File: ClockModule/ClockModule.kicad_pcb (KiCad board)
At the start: 2 copper layers, 93.5 x 65.5 mm, 34 parts, among them J1 Conn_01x05_Pin, SW1 SW_SPDT, U1 LM555xN, U2 LM555xN, U3 OR, U4 NOT, U6 LM555xN

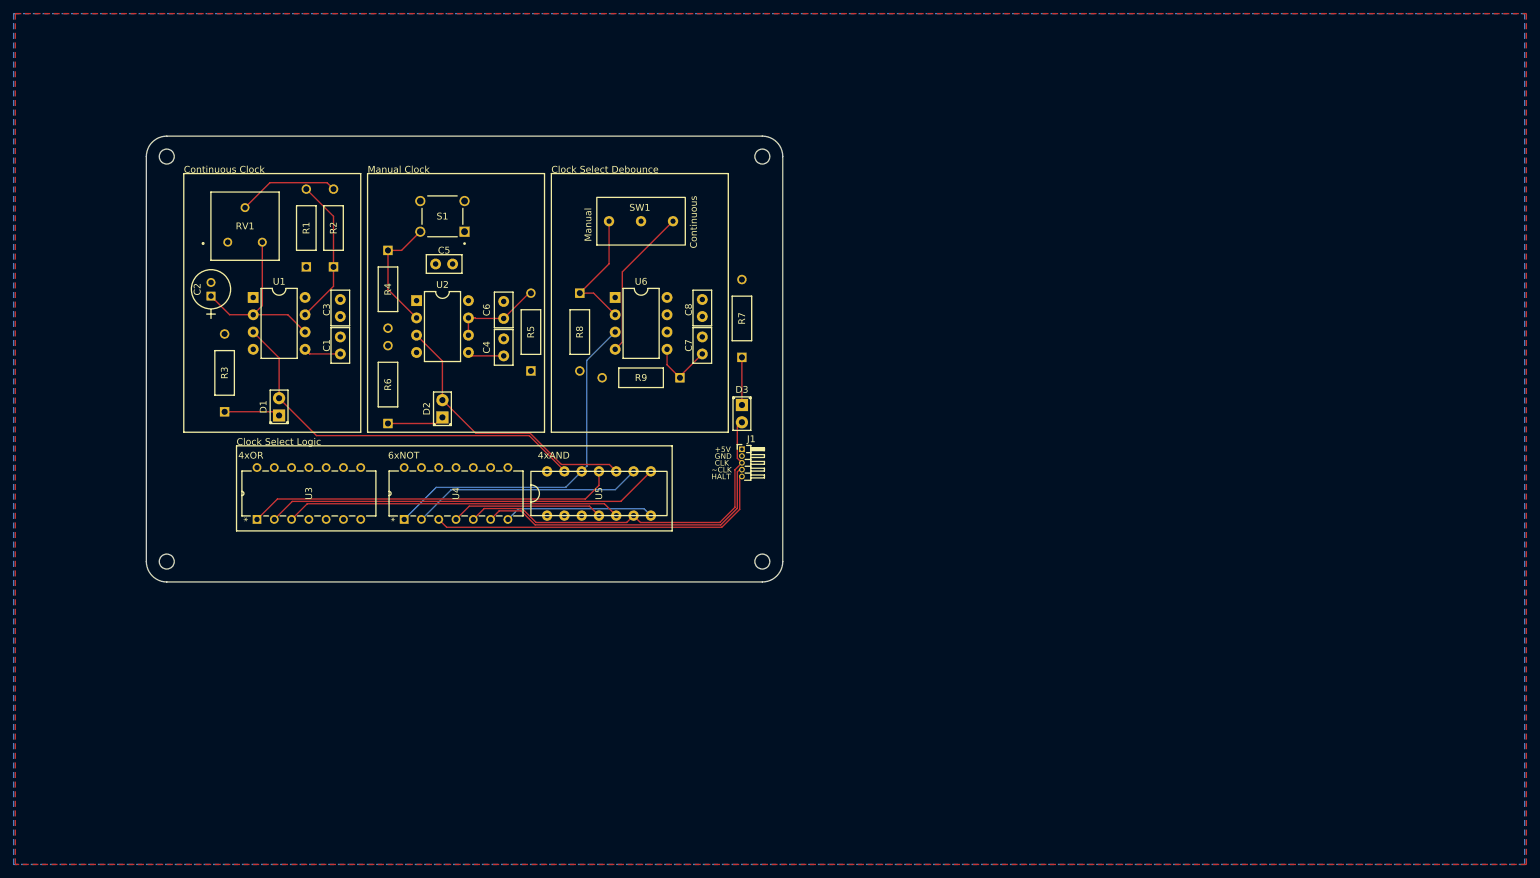
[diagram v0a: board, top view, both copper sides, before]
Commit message: Final clock updates
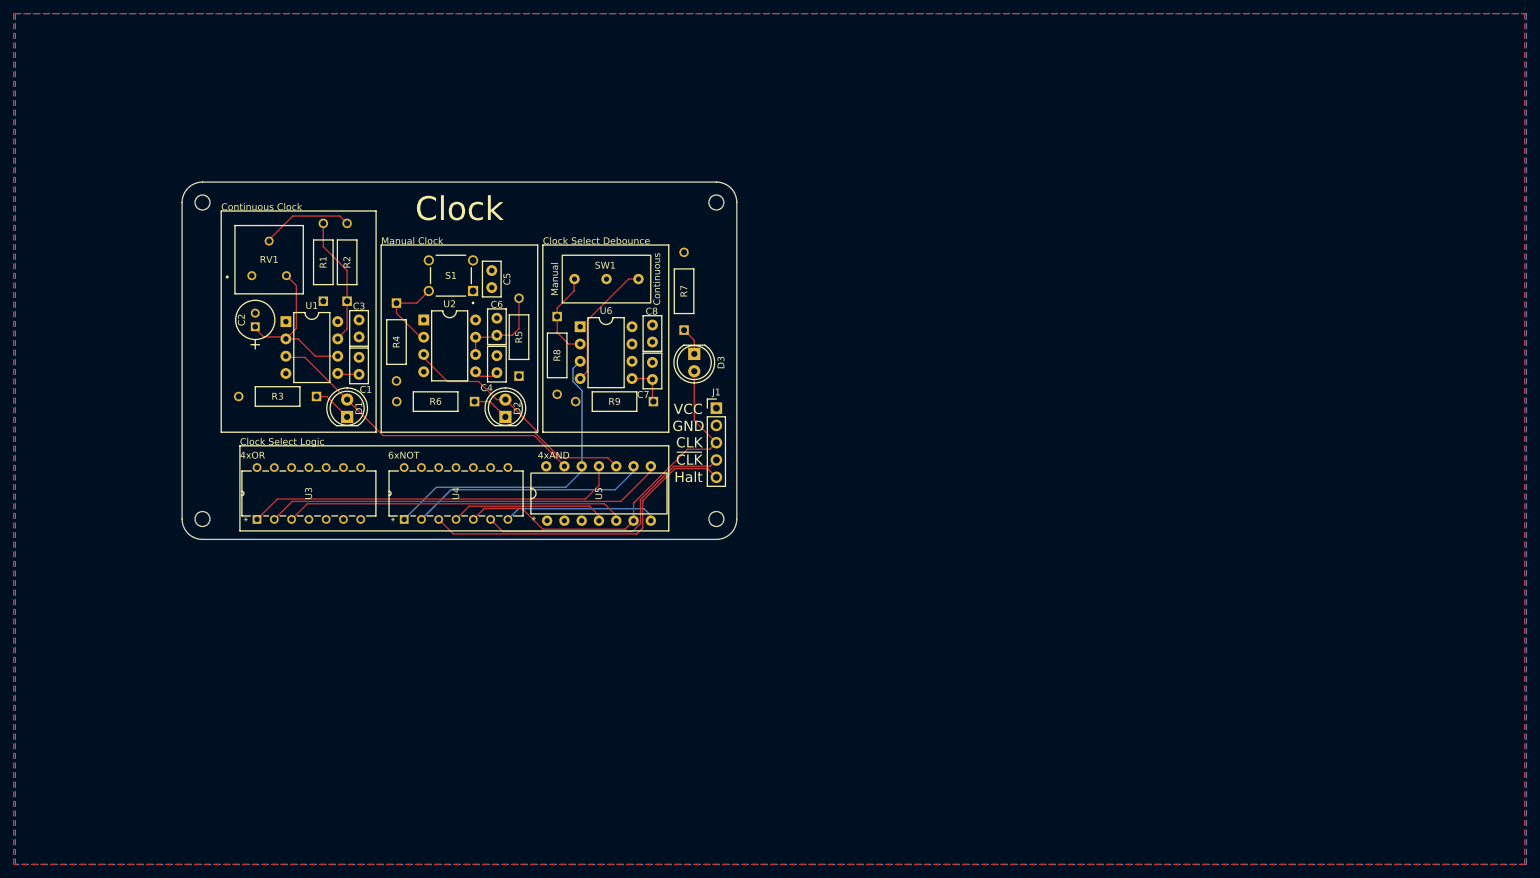
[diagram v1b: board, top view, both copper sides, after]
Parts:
- D1, D2, D3: footprint LED_THT:LED_D2.0mm_W4.8mm_H2.5mm_FlatTop -> LED_THT:LED_D5.0mm
- J1: footprint Connector_PinHeader_1.00mm:PinHeader_1x05_P1.00mm_Horizontal -> Connector_PinHeader_2.54mm:PinHeader_1x05_P2.54mm_Vertical
- moved R3 13.7 mm to (77.5, 102.8), turned to 180 degrees
- moved R6 13.1 mm to (100.7, 103.5), turned to 180 degrees
- moved D3 10.3 mm to (133.0, 96.5)
- moved D1 10.0 mm to (82.0, 105.8)
- moved SW1 9.90 mm to (120.1, 85.5)
- moved REF** 9.55 mm to (136.2, 74.2)
- moved R7 9.39 mm to (131.5, 93.0)
- moved D2 9.25 mm to (105.2, 105.8)
- moved REF** 9.20 mm to (136.2, 120.8)
- moved S1 8.80 mm to (97.2, 85.0)
- moved REF** 8.55 mm to (60.8, 74.2)
- moved C7 8.23 mm to (126.9, 100.2)
- moved C8 8.23 mm to (126.9, 92.2)
- moved REF** 8.16 mm to (60.8, 120.8)
- moved C2 7.91 mm to (68.5, 92.5)
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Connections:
- J1 pad 1: GND -> +5V
- J1 pad 2: +5V -> GND
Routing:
- net /AstableClock/CLK: track 57.7 -> 47.3 mm
- net Net-(SW1-A): track 18.9 -> 13.0 mm
- net /ClockSelect/BistableDebouncingCircuit/Select: track 51.5 -> 46.2 mm
- net /ClockSelect/Manual_clk: track 41.0 -> 35.7 mm
- net Net-(U2-TR): track 17.5 -> 12.4 mm
- net /~{clk}: track 44.8 -> 40.3 mm
- net Net-(SW1-C): track 22.3 -> 19.0 mm
- net Net-(U6-CV): track 9.83 -> 6.60 mm
- net Net-(D2-K): track 8.37 -> 5.47 mm
- net Net-(D3-K): track 7.00 -> 4.12 mm
- net Net-(U1-DIS): track 21.8 -> 19.0 mm
- net Net-(U1-THR): track 27.2 -> 24.6 mm
- net Net-(D1-K): track 8.22 -> 5.74 mm
- net Net-(U1-CV): track 5.46 -> 3.18 mm
- net /halt: track 50.7 -> 48.5 mm
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- added copper zone on F.Cu, net +5V
- added copper zone on B.Cu, net GND
- removed copper zone on B.Cu, net +5V
- removed copper zone on F.Cu, net GND
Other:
- board size 93.5 x 65.5 mm -> 81.5 x 52.5 mm
- board text added: "Clock"
- board text added: "Halt"
- board text added: "VCC"
- board text added: "~{CLK}"
- board text removed: "+5V"
- board text removed: "HALT"
- board text removed: "TODO: Double check 4xAND footprint"
- board text removed: "TODO: Figure out if I need more clock pins 1 for each module? Or just add it to the bus module and pass it around there?"
- board text removed: "~CLK"
